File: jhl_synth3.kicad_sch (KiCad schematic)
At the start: 14 parts, among them J1 Conn_01x05, J3 Conn_01x05, J4 DIN-5, J5 Conn_01x08, Q1 NPN 2N3904 SOT-23, Q2 NPN 2SC4116 SC-70, SW1 SW_Push, SW2 SW_Push, U1 YAAJ_WeAct_BlackPill_Part_Like, U2 TLP127

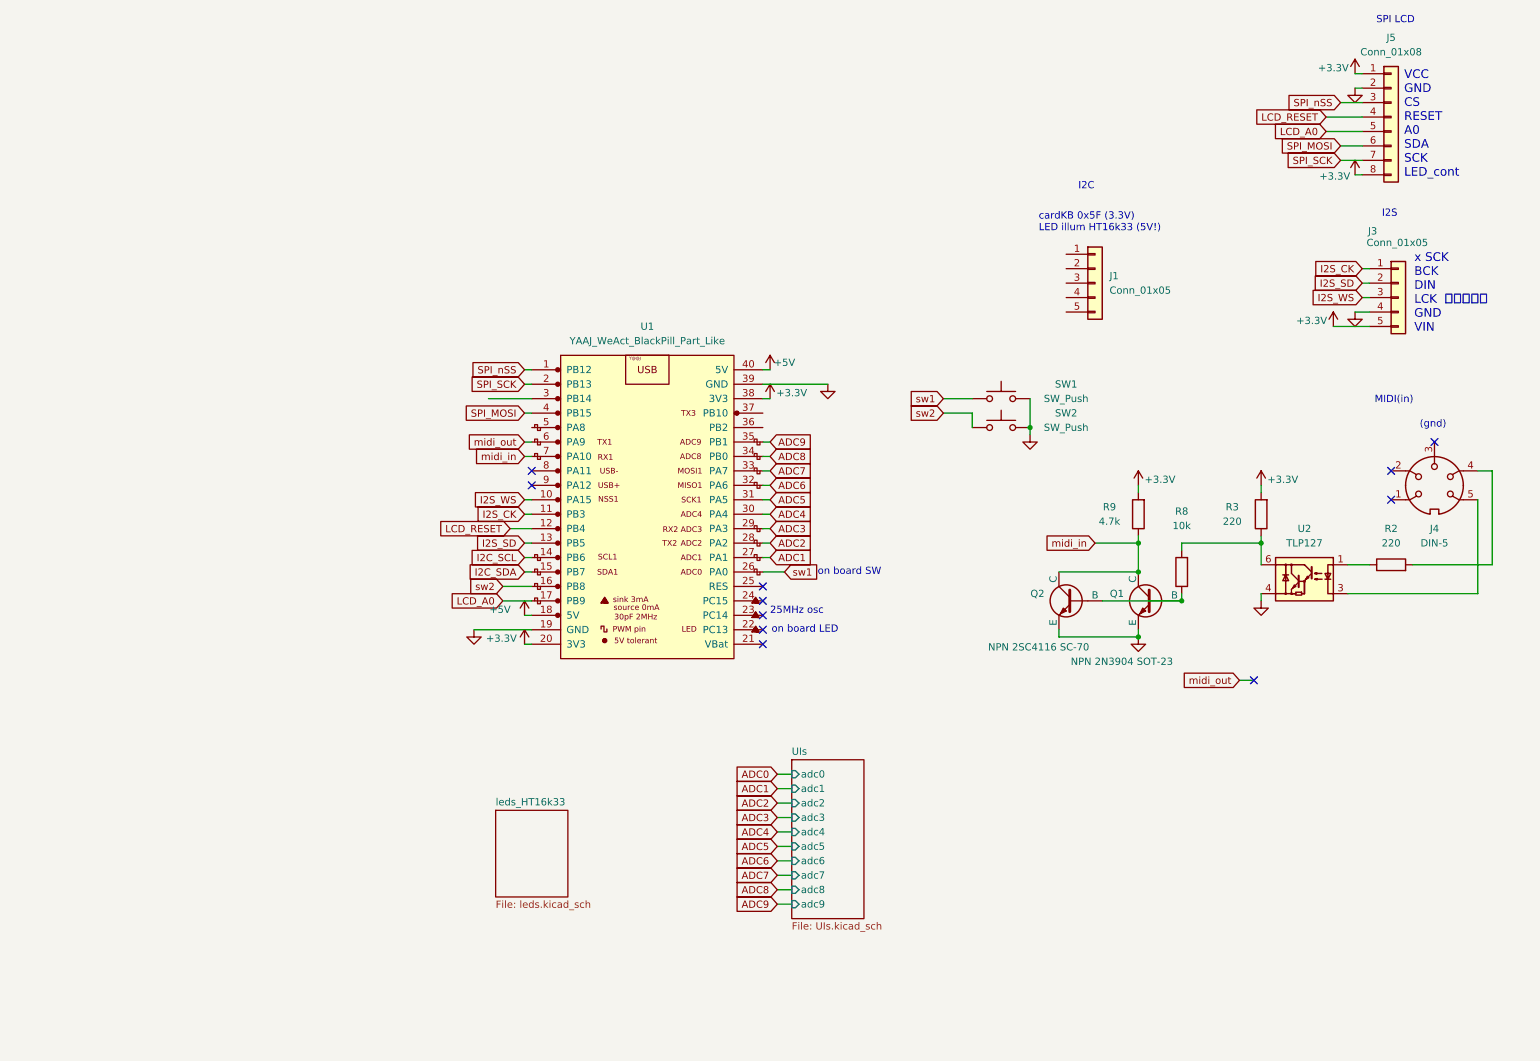
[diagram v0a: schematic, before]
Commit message: 定時
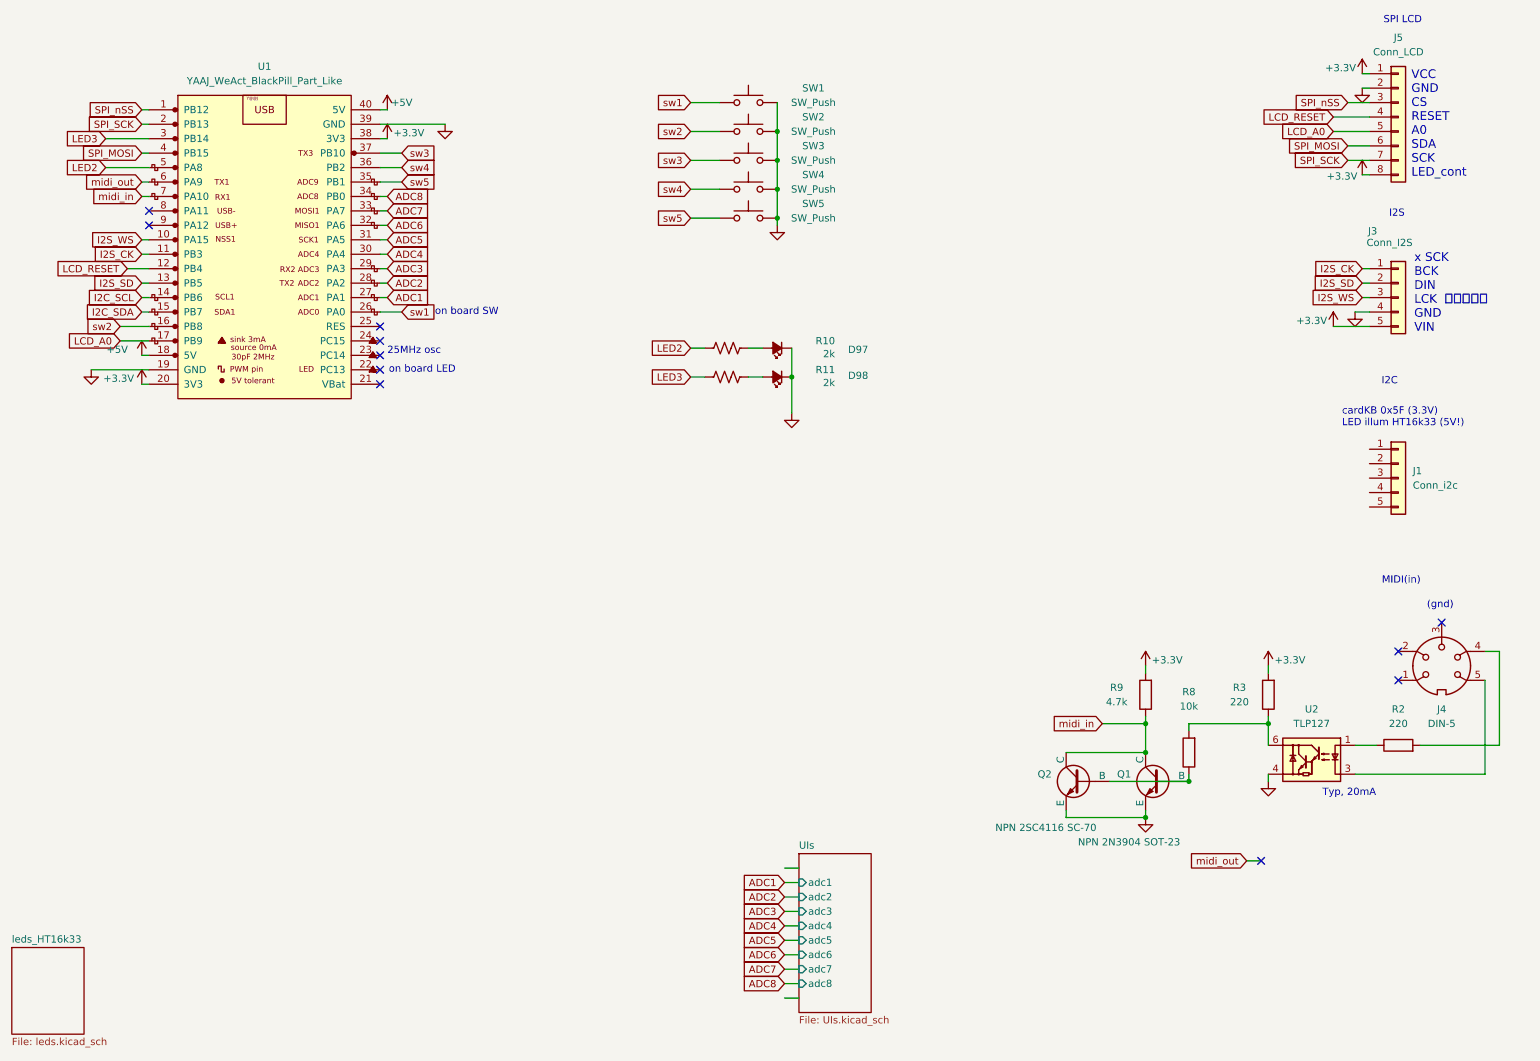
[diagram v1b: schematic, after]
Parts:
- added D97, D98: LED_Small_Filled, LED_SMD:LED_0603_1608Metric_Pad1.05x0.95mm_HandSolder, symbol Device:LED_Small_Filled
- added R10, R11: 2k, symbol Device:R_US
- added SW3, SW4, SW5: SW_Push, symbol Switch:SW_Push
- J1: value Conn_01x05 -> Conn_i2c
- J3: value Conn_01x05 -> Conn_I2S
- J5: value Conn_01x08 -> Conn_LCD
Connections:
- net GND: now also D97.1 (K), D98.1 (K), SW3.2, SW4.2, SW5.2
- net LED3: now reaches U1.3 (PB14)
- net LED3: now also R11.1
- net sw4: now reaches U1.36 (PB2)
- net sw4: now also SW4.1
- net sw3: now reaches U1.37 (PB10)
- net sw3: now also SW3.1
- net LED2: now reaches U1.5 (PA8)
- net LED2: now also R10.1
- net ADC9 renamed sw5
- net sw5: now also SW5.1
- new net: D98.2 (A), R11.2
- new net: D97.2 (A), R10.2
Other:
- sheet UIs ports: added none; removed adc0, adc9
- note added: "Typ, 20mA"
- moved on the sheet: J1, J4, J5, Q1, Q2, R2, R3, R8, R9, SW1, SW2, U1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
